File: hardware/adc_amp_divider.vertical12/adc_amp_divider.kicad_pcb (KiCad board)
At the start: 2 copper layers, 67.9 x 59.1 mm, 117 parts, among them M200 CONN_1, M201 CONN_1, M202 CONN_1, P201 CONN_10X2, P202 CONN_3, P203 CONN_2, P204 CONN_1, P205 CONN_1, P208 CONN_6, P209 CONN_6, U201 LMV324IDR, U202 LMV324IDR, U203 LMV324IDR

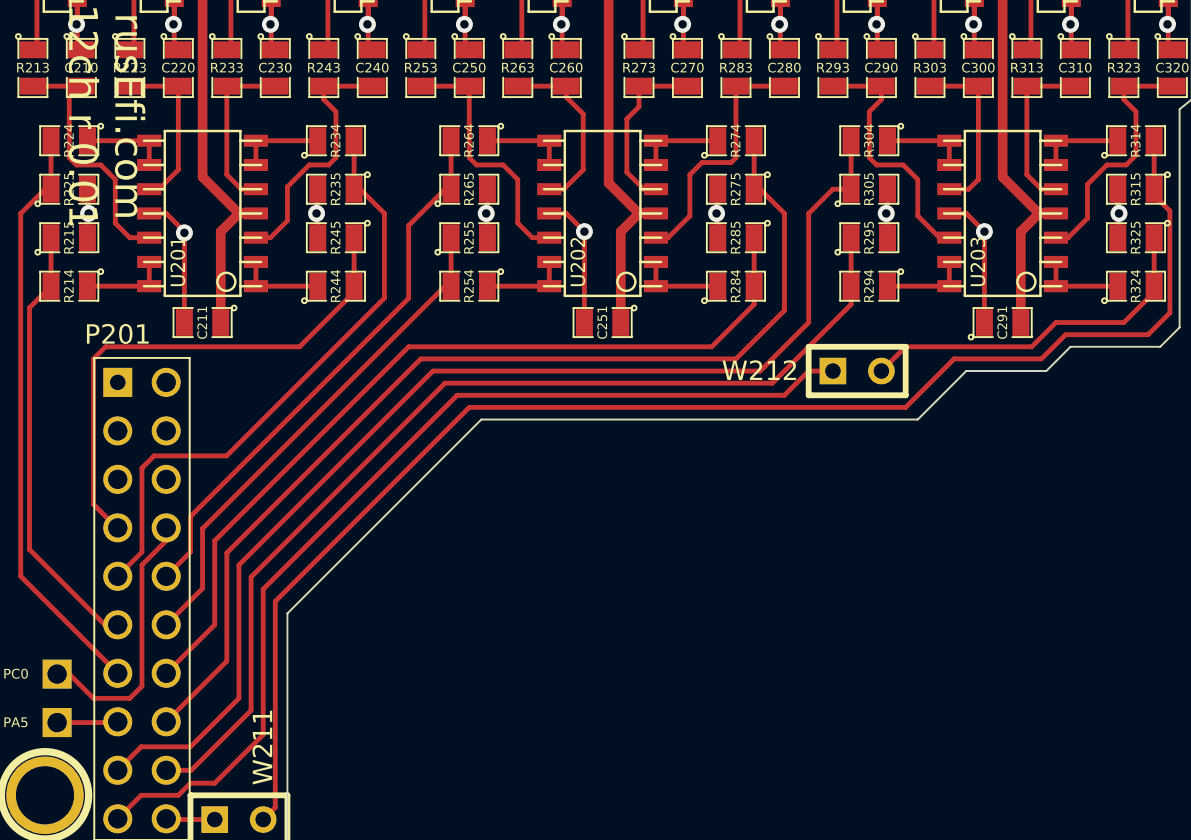
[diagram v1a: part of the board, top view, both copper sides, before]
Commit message: manual sync
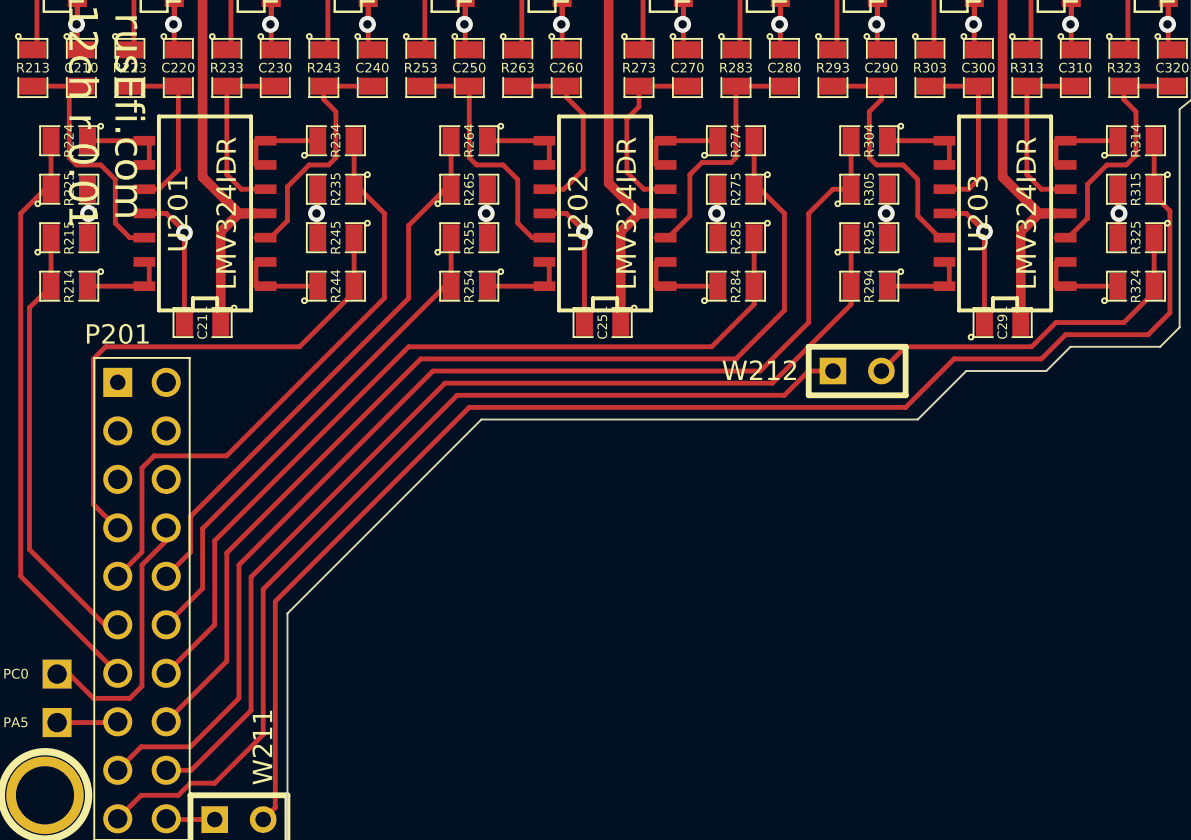
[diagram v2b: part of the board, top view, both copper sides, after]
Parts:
- U201, U202, U203: footprint so-14 -> SO14N
